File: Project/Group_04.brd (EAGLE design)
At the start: 29 parts, among them J1 POWER_JACKPTH_LOCK, U1 +12v

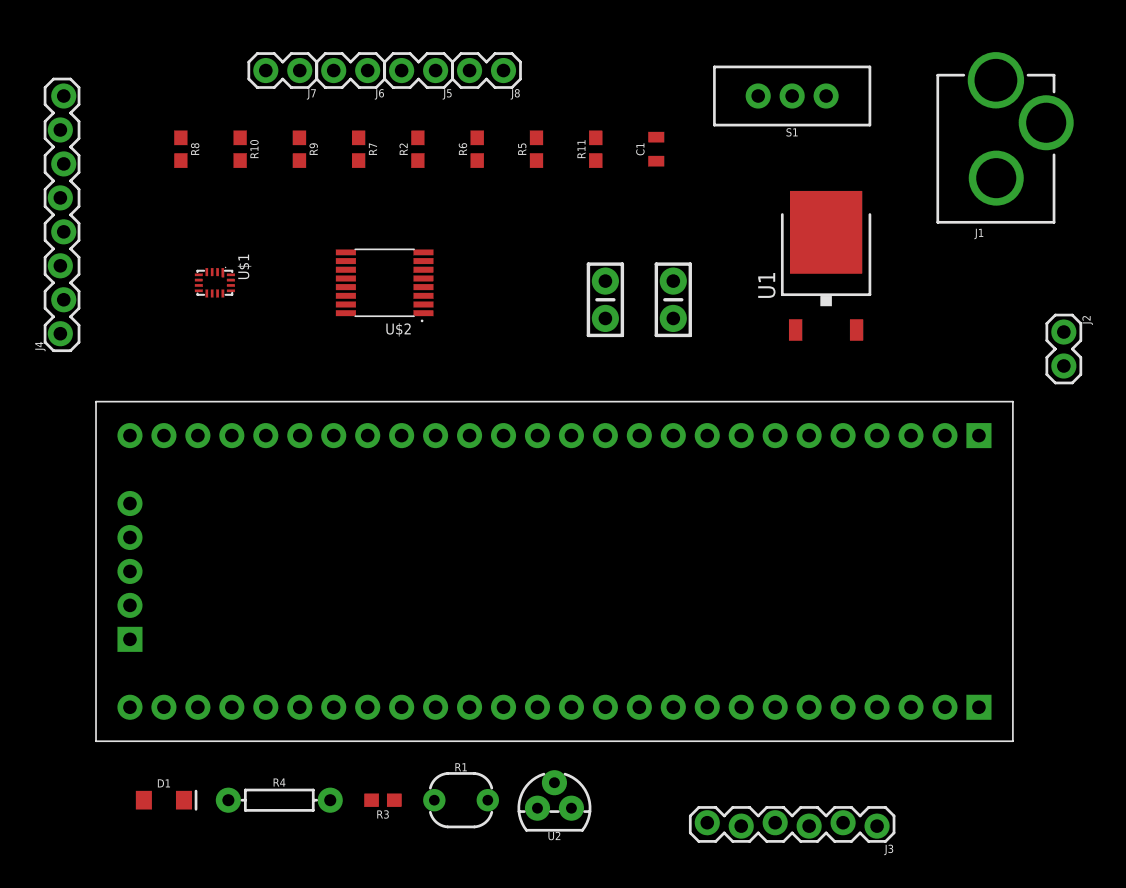
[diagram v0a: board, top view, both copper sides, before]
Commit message: routed
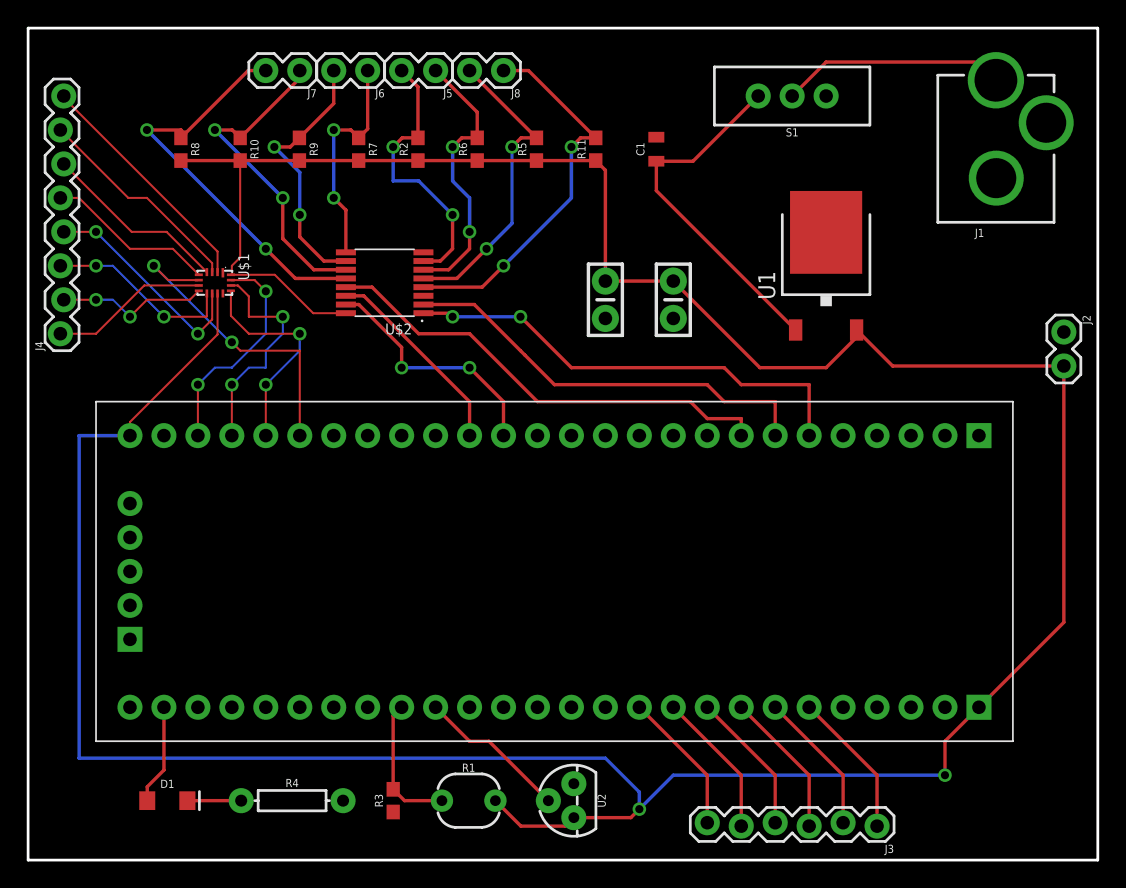
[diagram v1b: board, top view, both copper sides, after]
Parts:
- moved U2 1.56 mm to (40.8, 4.44), turned to 90 degrees
- moved R4 0.96 mm to (19.7, 4.44)
- moved R3 0.76 mm to (27.3, 4.44), turned to 90 degrees
- moved R1 0.57 mm to (33.0, 4.44)
- moved D1 0.26 mm to (10.4, 4.44)
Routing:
- net 5V: track 0.00 -> 254.5 mm, vias 0 -> 2
- net I2C_A2: track 0.00 -> 34.9 mm
- net I2C_A0: track 0.00 -> 34.9 mm, vias 0 -> 2
- net I2C_A1: track 0.00 -> 31.9 mm
- net I2C_SCL_3: track 0.00 -> 30.9 mm, vias 0 -> 2
- net I2C_SDA_0: track 0.00 -> 28.7 mm, vias 0 -> 2
- net 12V: track 0.00 -> 26.6 mm
- net I2C_SDA_3: track 0.00 -> 24.9 mm, vias 0 -> 2
- net MUX_OUT: track 0.00 -> 23.7 mm, vias 0 -> 2
- net I2C_SCL_0: track 0.00 -> 23.3 mm, vias 0 -> 2
- net I2C_SCL_1: track 0.00 -> 20.8 mm, vias 0 -> 2
- net I2C_SDA_1: track 0.00 -> 20.7 mm, vias 0 -> 2
- net I2C_SCL_2: track 0.00 -> 20.0 mm, vias 0 -> 2
- net I2C_SDA: track 0.00 -> 18.2 mm, vias 0 -> 2
- net N$10: track 0.00 -> 17.9 mm
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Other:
- board outline added: 80 x 62.2 mm
